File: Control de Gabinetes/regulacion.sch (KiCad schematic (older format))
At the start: 7 parts

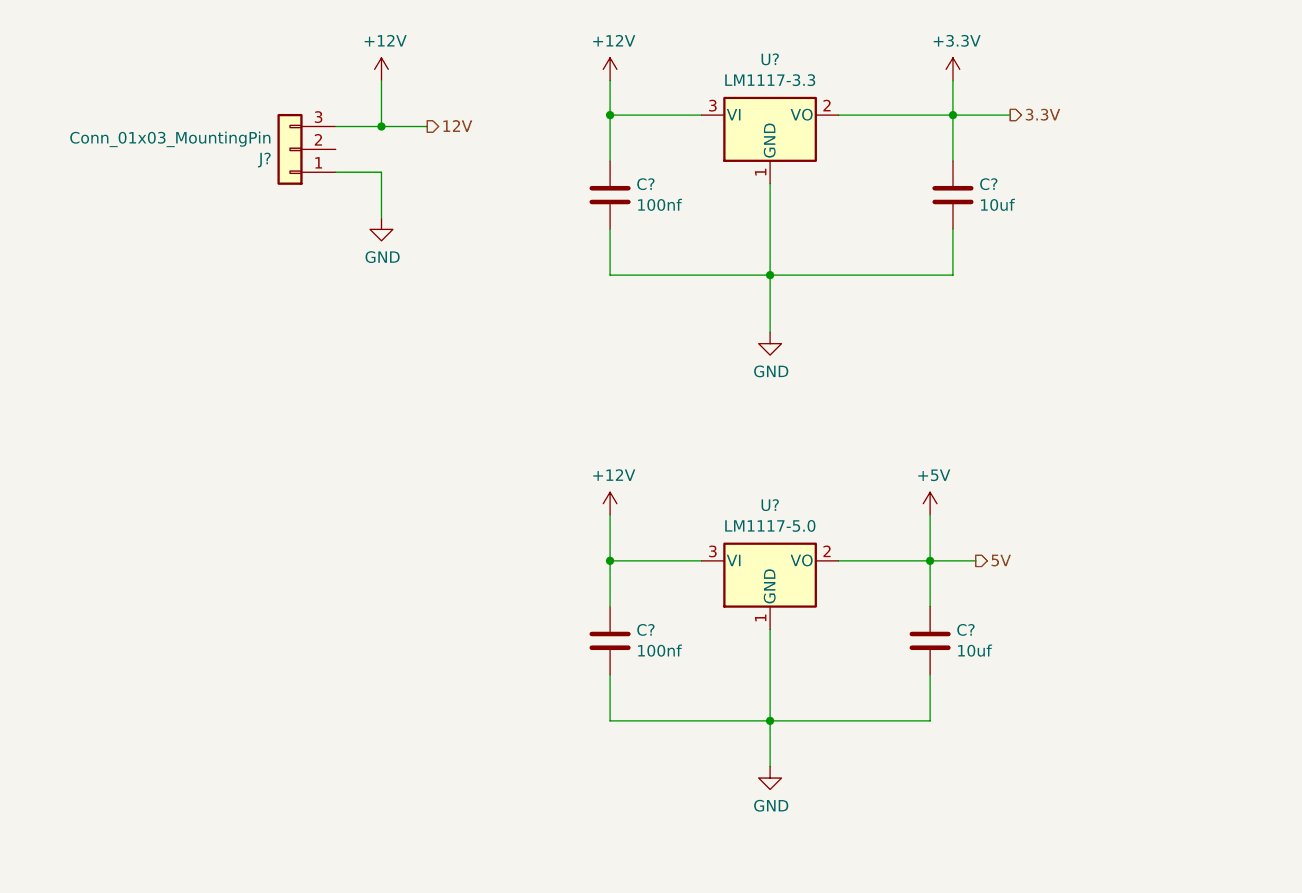
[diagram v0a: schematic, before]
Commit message: Avance 1/07/2021
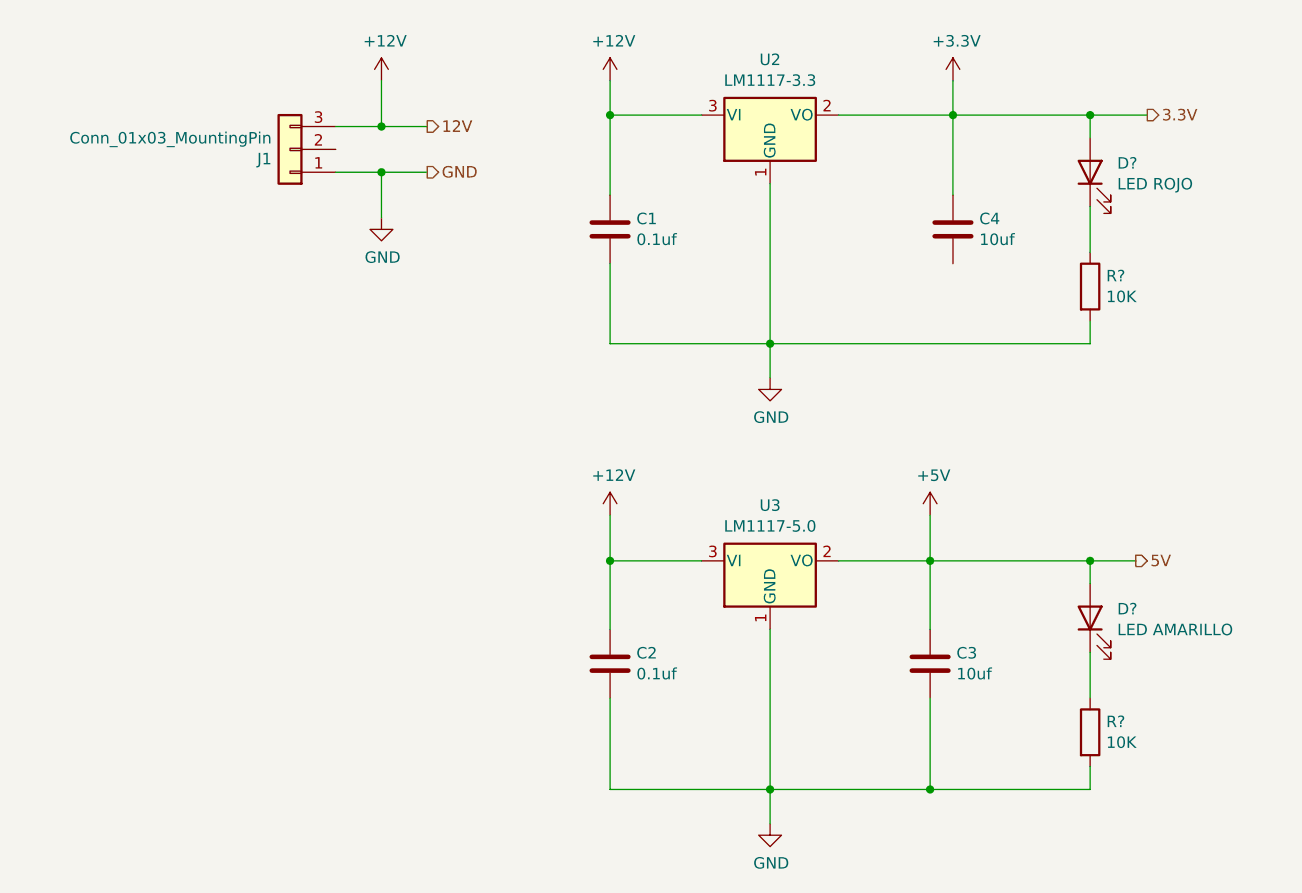
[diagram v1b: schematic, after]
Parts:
- added D?: LED ROJO, LED_SMD:LED_0805_2012Metric, symbol Device:LED
- added D?: LED AMARILLO, LED_SMD:LED_0805_2012Metric, symbol Device:LED
- added R? (x2): 10K, Resistor_SMD:R_0805_2012Metric, symbol Device:R
- C1, C2: renamed from C?; value 100nf -> 0.1uf
- gave numbers to parts that had none: 5
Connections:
- net +3V3: now also D?.2 (A)
- net +5V: now also D?.2 (A)
- net GND: now also R?.2, R?.2; no longer C4.2
- new net: D?.1 (K), R?.1 (x2)
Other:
- moved on the sheet: C1, C2, C3, C4
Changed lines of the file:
@@
 $EndDescr
 $Comp
-L Regulator_Linear:LM1117-3.3 U?
+L Regulator_Linear:LM1117-3.3 U2
 U 1 1 60989963
 P 3800 1350
-F 0 "U?" H 3800 1592 50  0000 C CNN
+F 0 "U2" H 3800 1592 50  0000 C CNN
 F 1 "LM1117-3.3" H 3800 1501 50  0000 C CNN
 F 2 "Package_TO_SOT_SMD:SOT-223-3_TabPin2" H 3800 1350 50  0001 C CNN
@@
 $EndComp
 $Comp
-L Regulator_Linear:LM1117-5.0 U?
+L Regulator_Linear:LM1117-5.0 U3
 U 1 1 6098A9C0
 P 3800 3300
-F 0 "U?" H 3800 3542 50  0000 C CNN
+F 0 "U3" H 3800 3542 50  0000 C CNN
 F 1 "LM1117-5.0" H 3800 3451 50  0000 C CNN
 F 2 "Package_TO_SOT_SMD:SOT-223-3_TabPin2" H 3800 3300 50  0001 C CNN
@@
 $EndComp
 $Comp
-L power:+3.3V #PWR?
+L power:+3.3V #PWR0106
 U 1 1 6098BC81
 P 4600 1200
-F 0 "#PWR?" H 4600 1050 50  0001 C CNN
+F 0 "#PWR0106" H 4600 1050 50  0001 C CNN
 F 1 "+3.3V" H 4615 1373 50  0000 C CNN
 F 2 "" H 4600 1200 50  0001 C CNN
@@
 $EndComp
 $Comp
-L power:GND #PWR?
+L power:GND #PWR0107
 U 1 1 6098C1DE
-P 3800 2300
-F 0 "#PWR?" H 3800 2050 50  0001 C CNN
-F 1 "GND" H 3805 2127 50  0000 C CNN
-F 2 "" H 3800 2300 50  0001 C CNN
-F 3 "" H 3800 2300 50  0001 C CNN
-	1    3800 2300
-	1    0    0    -1
-$EndComp
-$Comp
-L power:GND #PWR?
+P 3800 2500
+F 0 "#PWR0107" H 3800 2250 50  0001 C CNN
+F 1 "GND" H 3805 2327 50  0000 C CNN
+F 2 "" H 3800 2500 50  0001 C CNN
+F 3 "" H 3800 2500 50  0001 C CNN
+	1    3800 2500
+	1    0    0    -1
+$EndComp
+$Comp
+L power:GND #PWR0108
 U 1 1 6098C62D
-P 3800 4200
-F 0 "#PWR?" H 3800 3950 50  0001 C CNN
-F 1 "GND" H 3805 4027 50  0000 C CNN
-F 2 "" H 3800 4200 50  0001 C CNN
-F 3 "" H 3800 4200 50  0001 C CNN
-	1    3800 4200
-	1    0    0    -1
-$EndComp
-$Comp
-L power:+12V #PWR?
+P 3800 4450
+F 0 "#PWR0108" H 3800 4200 50  0001 C CNN
+F 1 "GND" H 3805 4277 50  0000 C CNN
+F 2 "" H 3800 4450 50  0001 C CNN
+F 3 "" H 3800 4450 50  0001 C CNN
+	1    3800 4450
+	1    0    0    -1
+$EndComp
+$Comp
+L power:+12V #PWR0109
 U 1 1 6098D21D
 P 3100 1200
-F 0 "#PWR?" H 3100 1050 50  0001 C CNN
+F 0 "#PWR0109" H 3100 1050 50  0001 C CNN
 F 1 "+12V" H 3115 1373 50  0000 C CNN
 F 2 "" H 3100 1200 50  0001 C CNN
@@
 $EndComp
 $Comp
-L power:+12V #PWR?
+L power:+12V #PWR0110
 U 1 1 6098DA98
 P 3100 3100
-F 0 "#PWR?" H 3100 2950 50  0001 C CNN
+F 0 "#PWR0110" H 3100 2950 50  0001 C CNN
 F 1 "+12V" H 3115 3273 50  0000 C CNN
 F 2 "" H 3100 3100 50  0001 C CNN
@@
 	3100 1350 3500 1350
 $Comp
-L Device:C C?
+L Device:C C1
 U 1 1 6099456B
-P 3100 1700
-F 0 "C?" H 3215 1746 50  0000 L CNN
-F 1 "100nf" H 3215 1655 50  0000 L CNN
-F 2 "Capacitor_SMD:C_0805_2012Metric" H 3138 1550 50  0001 C CNN
-F 3 "~" H 3100 1700 50  0001 C CNN
-	1    3100 1700
-	1    0    0    -1
-$EndComp
-Wire Wire Line
-	3100 1550 3100 1350
+P 3100 1850
+F 0 "C1" H 3215 1896 50  0000 L CNN
+F 1 "0.1uf" H 3215 1805 50  0000 L CNN
+F 2 "Capacitor_SMD:C_0805_2012Metric" H 3138 1700 50  0001 C CNN
+F 3 "~" H 3100 1850 50  0001 C CNN
+	1    3100 1850
+	1    0    0    -1
+$EndComp
 Connection ~ 3100 1350
-Wire Wire Line
-	3100 1850 3100 2050
-Wire Wire Line
-	3100 2050 3800 2050
-Wire Wire Line
-	3800 1650 3800 2050
-$Comp
-L Device:C C?
+$Comp
+L Device:C C4
 U 1 1 60997875
-P 4600 1700
-F 0 "C?" H 4715 1746 50  0000 L CNN
-F 1 "10uf" H 4715 1655 50  0000 L CNN
-F 2 "Capacitor_SMD:C_0805_2012Metric" H 4638 1550 50  0001 C CNN
-F 3 "~" H 4600 1700 50  0001 C CNN
-	1    4600 1700
-	1    0    0    -1
-$EndComp
-Wire Wire Line
-	4600 1850 4600 2050
-Wire Wire Line
-	4600 2050 3800 2050
-Connection ~ 3800 2050
-Wire Wire Line
-	3800 2300 3800 2050
-Wire Wire Line
-	4600 1550 4600 1350
+P 4600 1850
+F 0 "C4" H 4715 1896 50  0000 L CNN
+F 1 "10uf" H 4715 1805 50  0000 L CNN
+F 2 "Capacitor_SMD:C_0805_2012Metric" H 4638 1700 50  0001 C CNN
+F 3 "~" H 4600 1850 50  0001 C CNN
+	1    4600 1850
+	1    0    0    -1
+$EndComp
 Connection ~ 4600 1350
 $Comp
-L Device:C C?
+L Device:C C2
 U 1 1 60998C12
-P 3100 3650
-F 0 "C?" H 3215 3696 50  0000 L CNN
-F 1 "100nf" H 3215 3605 50  0000 L CNN
-F 2 "Capacitor_SMD:C_0805_2012Metric" H 3138 3500 50  0001 C CNN
-F 3 "~" H 3100 3650 50  0001 C CNN
-	1    3100 3650
-	1    0    0    -1
-$EndComp
-$Comp
-L Device:C C?
-U 1 1 60999295
-P 4500 3650
-F 0 "C?" H 4615 3696 50  0000 L CNN
-F 1 "10uf" H 4615 3605 50  0000 L CNN
-F 2 "Capacitor_SMD:C_0805_2012Metric" H 4538 3500 50  0001 C CNN
-F 3 "~" H 4500 3650 50  0001 C CNN
-	1    4500 3650
-	1    0    0    -1
-$EndComp
-Wire Wire Line
-	3100 3800 3100 4000
-Wire Wire Line
-	3100 4000 3800 4000
-Wire Wire Line
-	3800 3600 3800 4000
-Wire Wire Line
-	4500 3800 4500 4000
-Wire Wire Line
-	4500 4000 3800 4000
-Connection ~ 3800 4000
-Wire Wire Line
-	4500 3500 4500 3300
-Connection ~ 4500 3300
-Wire Wire Line
-	3100 3500 3100 3300
-Connection ~ 3100 3300
-Wire Wire Line
-	3800 4200 3800 4000
-Text HLabel 4850 1350 2    50   Output ~ 0
+P 3100 3750
+F 0 "C2" H 3215 3796 50  0000 L CNN
+F 1 "0.1uf" H 3215 3705 50  0000 L CNN
+F 2 "Capacitor_SMD:C_0805_2012Metric" H 3138 3600 50  0001 C CNN
+F 3 "~" H 3100 3750 50  0001 C CNN
+	1    3100 3750
+	1    0    0    -1
+$EndComp
+Text HLabel 5450 1350 2    50   Output ~ 0
 3.3V
 Wire Wire Line
-	4600 1350 4850 1350
-Text HLabel 4700 3300 2    50   Output ~ 0
+	5200 1350 5450 1350
+Text HLabel 5400 3300 2    50   Output ~ 0
 5V
 Wire Wire Line
-	4500 3300 4700 3300
-$Comp
-L power:+5V #PWR?
+	5200 3300 5400 3300
+$Comp
+L power:+5V #PWR0111
 U 1 1 6099CBA4
 P 4500 3100
-F 0 "#PWR?" H 4500 2950 50  0001 C CNN
+F 0 "#PWR0111" H 4500 2950 50  0001 C CNN
 F 1 "+5V" H 4515 3273 50  0000 C CNN
 F 2 "" H 4500 3100 50  0001 C CNN
@@
 $EndComp
 $Comp
-L Connector_Generic:Conn_01x03 J?
+L Connector_Generic:Conn_01x03 J1
 U 1 1 609AC590
 P 1700 1500
-F 0 "J?" H 1780 1542 50  0000 L CNN
+F 0 "J1" H 1780 1542 50  0000 L CNN
 F 1 "Conn_01x03_MountingPin" H 1780 1451 50  0000 L CNN
 F 2 "Connector_Molex:Molex_KK-254_AE-6410-03A_1x03_P2.54mm_Vertical" H 1700 1500 50  0001 C CNN
@@
 $EndComp
 $Comp
-L power:+12V #PWR?
+L power:+12V #PWR0112
 U 1 1 609AF6B3
 P 2100 1200
-F 0 "#PWR?" H 2100 1050 50  0001 C CNN
+F 0 "#PWR0112" H 2100 1050 50  0001 C CNN
 F 1 "+12V" H 2115 1373 50  0000 C CNN
 F 2 "" H 2100 1200 50  0001 C CNN
@@
 $EndComp
 $Comp
-L power:GND #PWR?
+L power:GND #PWR0113
 U 1 1 609B0051
 P 2100 1800
-F 0 "#PWR?" H 2100 1550 50  0001 C CNN
+F 0 "#PWR0113" H 2100 1550 50  0001 C CNN
 F 1 "GND" H 2105 1627 50  0000 C CNN
 F 2 "" H 2100 1800 50  0001 C CNN
@@
 	2100 1400 2300 1400
 Connection ~ 2100 1400
+Text HLabel 2300 1600 2    50   Output ~ 0
+GND
+Wire Wire Line
+	2300 1600 2100 1600
+Connection ~ 2100 1600
+$Comp
+L Device:LED D?
+U 1 1 60E20F7B
+P 5200 1600
+F 0 "D?" V 5239 1482 50  0000 R CNN
+F 1 "LED ROJO" V 5148 1482 50  0000 R CNN
+F 2 "LED_SMD:LED_0805_2012Metric" H 5200 1600 50  0001 C CNN
+F 3 "~" H 5200 1600 50  0001 C CNN
+	1    5200 1600
+	0    -1   -1   0
+$EndComp
+$Comp
+L Device:R R?
+U 1 1 60E239E3
+P 5200 2100
+F 0 "R?" H 5270 2146 50  0000 L CNN
+F 1 "10K" H 5270 2055 50  0000 L CNN
+F 2 "Resistor_SMD:R_0805_2012Metric" V 5130 2100 50  0001 C CNN
+F 3 "~" H 5200 2100 50  0001 C CNN
+	1    5200 2100
+	1    0    0    -1
+$EndComp
+Wire Wire Line
+	4600 1350 4600 1700
+Wire Wire Line
+	3100 1350 3100 1700
+Wire Wire Line
+	5200 1750 5200 1950
+Wire Wire Line
+	5200 1450 5200 1350
+Wire Wire Line
+	5200 1350 4600 1350
+Connection ~ 5200 1350
+$Comp
+L Device:LED D?
+U 1 1 60E29EA4
+P 5200 3550
+F 0 "D?" V 5239 3432 50  0000 R CNN
+F 1 "LED AMARILLO" V 5148 3432 50  0000 R CNN
+F 2 "LED_SMD:LED_0805_2012Metric" H 5200 3550 50  0001 C CNN
+F 3 "~" H 5200 3550 50  0001 C CNN
+	1    5200 3550
+	0    -1   -1   0
+$EndComp
+$Comp
+L Device:R R?
+U 1 1 60E2A004
+P 5200 4050
+F 0 "R?" H 5270 4096 50  0000 L CNN
+F 1 "10K" H 5270 4005 50  0000 L CNN
+F 2 "Resistor_SMD:R_0805_2012Metric" V 5130 4050 50  0001 C CNN
+F 3 "~" H 5200 4050 50  0001 C CNN
+	1    5200 4050
+	1    0    0    -1
+$EndComp
+Wire Wire Line
+	5200 3700 5200 3900
+$Comp
+L Device:C C3
+U 1 1 60999295
+P 4500 3750
+F 0 "C3" H 4615 3796 50  0000 L CNN
+F 1 "10uf" H 4615 3705 50  0000 L CNN
+F 2 "Capacitor_SMD:C_0805_2012Metric" H 4538 3600 50  0001 C CNN
+F 3 "~" H 4500 3750 50  0001 C CNN
+	1    4500 3750
+	1    0    0    -1
+$EndComp
+Wire Wire Line
+	5200 2250 5200 2350
+Wire Wire Line
+	5200 2350 3800 2350
+Wire Wire Line
+	3100 2000 3100 2350
+Wire Wire Line
+	5200 4200 5200 4300
+Wire Wire Line
+	5200 4300 4500 4300
+Wire Wire Line
+	3100 4300 3100 3900
+Wire Wire Line
+	3100 3300 3100 3600
+Connection ~ 3100 3300
+Wire Wire Line
+	4500 3300 4500 3600
+Connection ~ 4500 3300
+Wire Wire Line
+	4500 3900 4500 4300
+Connection ~ 4500 4300
+Wire Wire Line
+	4500 4300 3800 4300
+Wire Wire Line
+	5200 3400 5200 3300
+Wire Wire Line
+	4500 3300 5200 3300
+Connection ~ 5200 3300
+Wire Wire Line
+	3800 1650 3800 2350
+Connection ~ 3800 2350
+Wire Wire Line
+	3800 2350 3100 2350
+Wire Wire Line
+	3800 2500 3800 2350
+Wire Wire Line
+	3800 3600 3800 4300
+Connection ~ 3800 4300
+Wire Wire Line
+	3800 4300 3100 4300
+Wire Wire Line
+	3800 4450 3800 4300
 $EndSCHEMATC

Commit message: avance 6/07
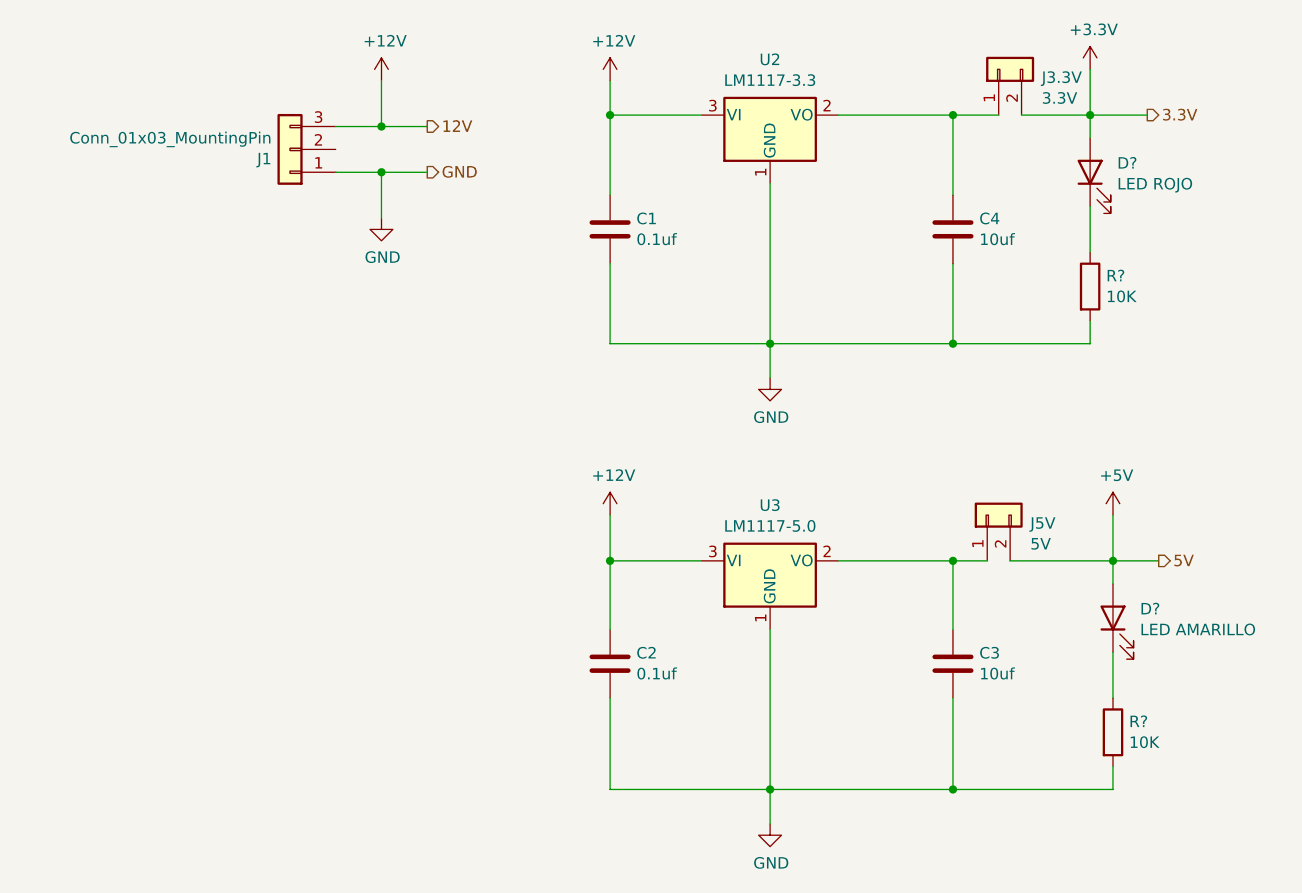
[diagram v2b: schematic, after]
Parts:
- added J3.3V: 3.3V, Connector_PinHeader_2.54mm:PinHeader_1x02_P2.54mm_Vertical, symbol Connector_Generic:Conn_01x02
- added J5V: 5V, Connector_PinHeader_2.54mm:PinHeader_1x02_P2.54mm_Vertical, symbol Connector_Generic:Conn_01x02
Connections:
- net +3V3: now also J3.3V.2 (Pin_2); no longer C4.1, U2.2 (VO)
- net +5V: now also J5V.2 (Pin_2); no longer C3.1, U3.2 (VO)
- net GND: now also C4.2
- new net: C4.1, J3.3V.1 (Pin_1), U2.2 (VO)
- new net: C3.1, J5V.1 (Pin_1), U3.2 (VO)
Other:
- moved on the sheet: C3, D?, R?
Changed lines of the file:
@@
 EELAYER 30 0
 EELAYER END
-$Descr A4 11693 8268
+$Descr User 7087 7087
 encoding utf-8
-Sheet 3 6
+Sheet 2 6
 Title ""
 Date ""
@@
 L power:+3.3V #PWR0106
 U 1 1 6098BC81
-P 4600 1200
-F 0 "#PWR0106" H 4600 1050 50  0001 C CNN
-F 1 "+3.3V" H 4615 1373 50  0000 C CNN
-F 2 "" H 4600 1200 50  0001 C CNN
-F 3 "" H 4600 1200 50  0001 C CNN
-	1    4600 1200
+P 5200 1150
+F 0 "#PWR0106" H 5200 1000 50  0001 C CNN
+F 1 "+3.3V" H 5215 1323 50  0000 C CNN
+F 2 "" H 5200 1150 50  0001 C CNN
+F 3 "" H 5200 1150 50  0001 C CNN
+	1    5200 1150
 	1    0    0    -1
 $EndComp
@@
 $EndComp
 Wire Wire Line
-	4100 1350 4600 1350
-Wire Wire Line
-	4600 1350 4600 1200
-Wire Wire Line
 	3100 1350 3100 1200
-Wire Wire Line
-	4100 3300 4500 3300
-Wire Wire Line
-	4500 3300 4500 3100
 Wire Wire Line
 	3500 3300 3100 3300
@@
 	1    0    0    -1
 $EndComp
-Connection ~ 4600 1350
 $Comp
 L Device:C C2
@@
 Wire Wire Line
 	5200 1350 5450 1350
-Text HLabel 5400 3300 2    50   Output ~ 0
+Text HLabel 5500 3300 2    50   Output ~ 0
 5V
 Wire Wire Line
-	5200 3300 5400 3300
+	5300 3300 5500 3300
 $Comp
 L power:+5V #PWR0111
 U 1 1 6099CBA4
-P 4500 3100
-F 0 "#PWR0111" H 4500 2950 50  0001 C CNN
-F 1 "+5V" H 4515 3273 50  0000 C CNN
-F 2 "" H 4500 3100 50  0001 C CNN
-F 3 "" H 4500 3100 50  0001 C CNN
-	1    4500 3100
+P 5300 3100
+F 0 "#PWR0111" H 5300 2950 50  0001 C CNN
+F 1 "+5V" H 5315 3273 50  0000 C CNN
+F 2 "" H 5300 3100 50  0001 C CNN
+F 3 "" H 5300 3100 50  0001 C CNN
+	1    5300 3100
 	1    0    0    -1
 $EndComp
@@
 Wire Wire Line
 	5200 1450 5200 1350
-Wire Wire Line
-	5200 1350 4600 1350
 Connection ~ 5200 1350
 $Comp
 L Device:LED D?
 U 1 1 60E29EA4
-P 5200 3550
-F 0 "D?" V 5239 3432 50  0000 R CNN
-F 1 "LED AMARILLO" V 5148 3432 50  0000 R CNN
-F 2 "LED_SMD:LED_0805_2012Metric" H 5200 3550 50  0001 C CNN
-F 3 "~" H 5200 3550 50  0001 C CNN
-	1    5200 3550
+P 5300 3550
+F 0 "D?" V 5339 3432 50  0000 R CNN
+F 1 "LED AMARILLO" V 5248 3432 50  0000 R CNN
+F 2 "LED_SMD:LED_0805_2012Metric" H 5300 3550 50  0001 C CNN
+F 3 "~" H 5300 3550 50  0001 C CNN
+	1    5300 3550
 	0    -1   -1   0
 $EndComp
@@
 L Device:R R?
 U 1 1 60E2A004
-P 5200 4050
-F 0 "R?" H 5270 4096 50  0000 L CNN
-F 1 "10K" H 5270 4005 50  0000 L CNN
-F 2 "Resistor_SMD:R_0805_2012Metric" V 5130 4050 50  0001 C CNN
-F 3 "~" H 5200 4050 50  0001 C CNN
-	1    5200 4050
-	1    0    0    -1
-$EndComp
-Wire Wire Line
-	5200 3700 5200 3900
+P 5300 4050
+F 0 "R?" H 5370 4096 50  0000 L CNN
+F 1 "10K" H 5370 4005 50  0000 L CNN
+F 2 "Resistor_SMD:R_0805_2012Metric" V 5230 4050 50  0001 C CNN
+F 3 "~" H 5300 4050 50  0001 C CNN
+	1    5300 4050
+	1    0    0    -1
+$EndComp
+Wire Wire Line
+	5300 3700 5300 3900
 $Comp
 L Device:C C3
 U 1 1 60999295
-P 4500 3750
-F 0 "C3" H 4615 3796 50  0000 L CNN
-F 1 "10uf" H 4615 3705 50  0000 L CNN
-F 2 "Capacitor_SMD:C_0805_2012Metric" H 4538 3600 50  0001 C CNN
-F 3 "~" H 4500 3750 50  0001 C CNN
-	1    4500 3750
+P 4600 3750
+F 0 "C3" H 4715 3796 50  0000 L CNN
+F 1 "10uf" H 4715 3705 50  0000 L CNN
+F 2 "Capacitor_SMD:C_0805_2012Metric" H 4638 3600 50  0001 C CNN
+F 3 "~" H 4600 3750 50  0001 C CNN
+	1    4600 3750
 	1    0    0    -1
 $EndComp
@@
 	5200 2250 5200 2350
 Wire Wire Line
-	5200 2350 3800 2350
+	5200 2350 4600 2350
 Wire Wire Line
 	3100 2000 3100 2350
 Wire Wire Line
-	5200 4200 5200 4300
-Wire Wire Line
-	5200 4300 4500 4300
+	5300 4200 5300 4300
+Wire Wire Line
+	5300 4300 4600 4300
 Wire Wire Line
 	3100 4300 3100 3900
@@
 Connection ~ 3100 3300
 Wire Wire Line
-	4500 3300 4500 3600
-Connection ~ 4500 3300
-Wire Wire Line
-	4500 3900 4500 4300
-Connection ~ 4500 4300
-Wire Wire Line
-	4500 4300 3800 4300
-Wire Wire Line
-	5200 3400 5200 3300
-Wire Wire Line
-	4500 3300 5200 3300
-Connection ~ 5200 3300
+	4600 3300 4600 3600
+Wire Wire Line
+	4600 3900 4600 4300
+Connection ~ 4600 4300
+Wire Wire Line
+	5300 3400 5300 3300
+Connection ~ 5300 3300
 Wire Wire Line
 	3800 1650 3800 2350
@@
 Wire Wire Line
 	3800 4450 3800 4300
+$Comp
+L Connector_Generic:Conn_01x02 J3.3V
+U 1 1 60E4AE87
+P 4800 1150
+F 0 "J3.3V" V 4764 962 50  0000 R CNN
+F 1 "3.3V" V 4673 962 50  0000 R CNN
+F 2 "Connector_PinHeader_2.54mm:PinHeader_1x02_P2.54mm_Vertical" H 4800 1150 50  0001 C CNN
+F 3 "~" H 4800 1150 50  0001 C CNN
+	1    4800 1150
+	0    -1   -1   0
+$EndComp
+Wire Wire Line
+	4600 2000 4600 2350
+Connection ~ 4600 2350
+Wire Wire Line
+	4600 2350 3800 2350
+Wire Wire Line
+	5200 1150 5200 1350
+Wire Wire Line
+	5300 3100 5300 3300
+$Comp
+L Connector_Generic:Conn_01x02 J5V
+U 1 1 60E51F0A
+P 4750 3100
+F 0 "J5V" V 4714 2912 50  0000 R CNN
+F 1 "5V" V 4623 2912 50  0000 R CNN
+F 2 "Connector_PinHeader_2.54mm:PinHeader_1x02_P2.54mm_Vertical" H 4750 3100 50  0001 C CNN
+F 3 "~" H 4750 3100 50  0001 C CNN
+F 4 "" V 4750 3100 50  0001 C CNN "Field4"
+	1    4750 3100
+	0    -1   -1   0
+$EndComp
+Wire Wire Line
+	3800 4300 4600 4300
+Wire Wire Line
+	4100 3300 4600 3300
+Wire Wire Line
+	4750 3300 4600 3300
+Connection ~ 4600 3300
+Wire Wire Line
+	4850 3300 5300 3300
+Wire Wire Line
+	4800 1350 4600 1350
+Wire Wire Line
+	4100 1350 4600 1350
+Connection ~ 4600 1350
+Wire Wire Line
+	4900 1350 5200 1350
 $EndSCHEMATC
